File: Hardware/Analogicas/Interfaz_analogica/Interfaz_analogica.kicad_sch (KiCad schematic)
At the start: 1 part, among them U1 LM741

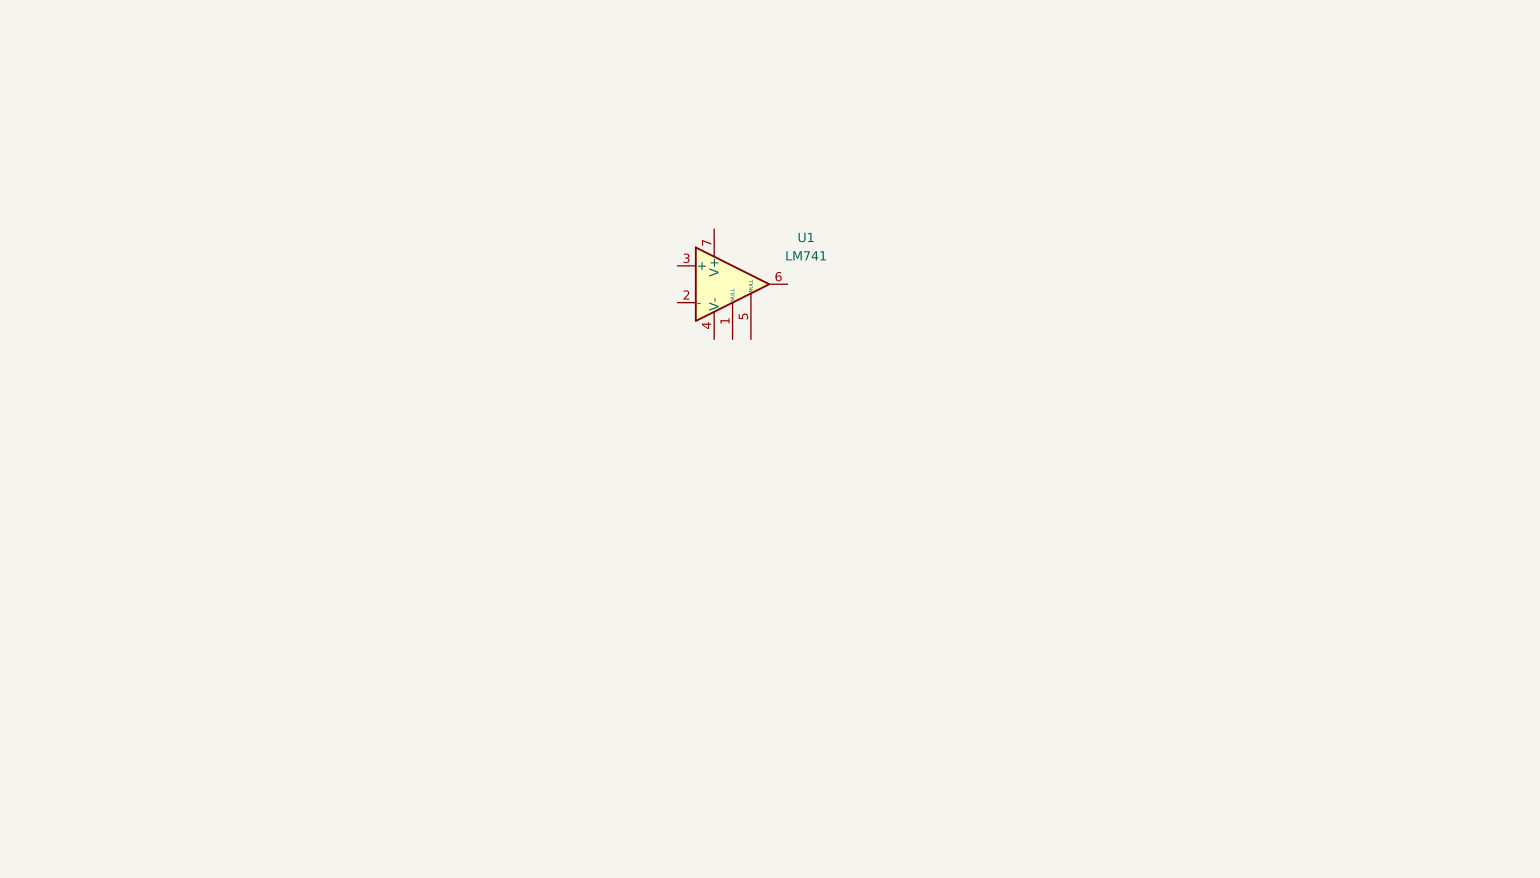
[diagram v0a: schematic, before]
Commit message: Interfaz analógica
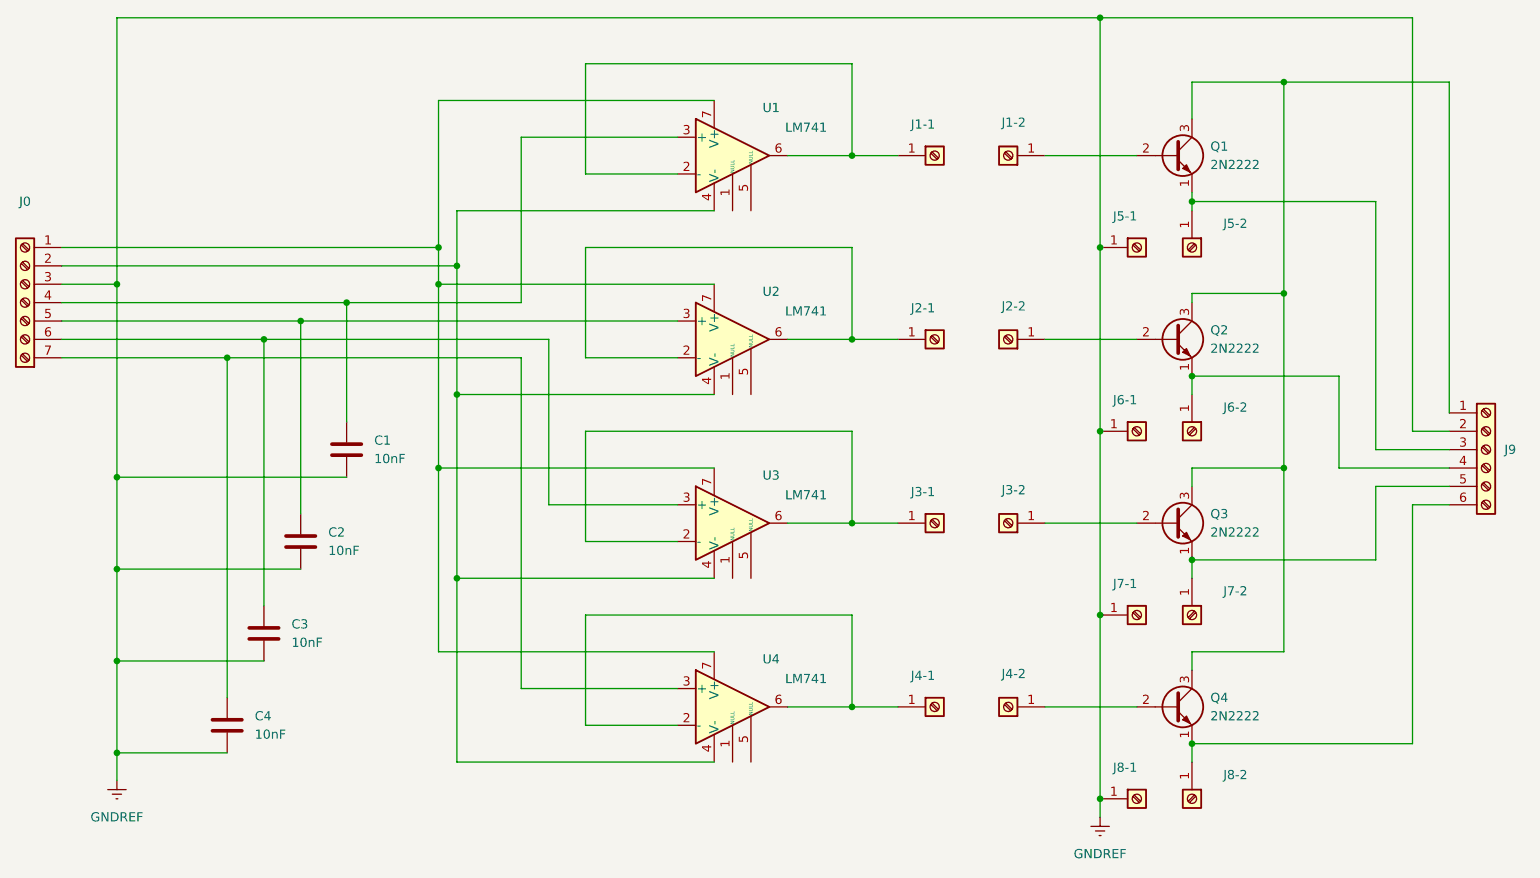
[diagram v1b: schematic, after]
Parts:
- added C1, C2, C3, C4: 10nF, symbol Device:C
- added J0: Screw_Terminal_01x07, symbol Connector:Screw_Terminal_01x07
- added J1-1, J1-2, J2-1, J2-2, J3-1, J3-2, J4-1, J4-2, J5-1, J5-2, J6-1, J6-2, J7-1, J7-2, J8-1, J8-2: Screw_Terminal_01x01, symbol Connector:Screw_Terminal_01x01
- added J9: Screw_Terminal_01x06, symbol Connector:Screw_Terminal_01x06
- added Q1, Q2, Q3, Q4: 2N2222, Package_TO_SOT_THT:TO-39-3, symbol Transistor_BJT:2N2219
- added U2, U3, U4: LM741, symbol Amplifier_Operational:LM741
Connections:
- net at U1.2 (-): now also U1.6, J1-1.1 (Pin_1)
- net at U1.3 (+): now also C1.1, J0.4 (Pin_4)
- net at U1.4 (V-): now also J0.2 (Pin_2), U2.4 (V-), U3.4 (V-), U4.4 (V-)
- net at U1.7 (V+): now also J0.1 (Pin_1), U2.7 (V+), U3.7 (V+), U4.7 (V+)
- new net: J6-2.1 (Pin_1), J9.4 (Pin_4), Q2.1 (E)
- new net: J7-2.1 (Pin_1), J9.5 (Pin_5), Q3.1 (E)
- new net: C3.1, J0.6 (Pin_6), U3.3 (+)
- new net: J3-1.1 (Pin_1), U3.2 (-), U3.6
- new net: J4-1.1 (Pin_1), U4.2 (-), U4.6
- new net: C4.1, J0.7 (Pin_7), U4.3 (+)
- new net: J2-1.1 (Pin_1), U2.2 (-), U2.6
- new net: C2.1, J0.5 (Pin_5), U2.3 (+)
- new net: J2-2.1 (Pin_1), Q2.2 (B)
- new net: J9.1 (Pin_1), Q1.3 (C), Q2.3 (C), Q3.3 (C), Q4.3 (C)
- new net: J5-2.1 (Pin_1), J9.3 (Pin_3), Q1.1 (E)
- new net: J8-2.1 (Pin_1), J9.6 (Pin_6), Q4.1 (E)
- new net: J4-2.1 (Pin_1), Q4.2 (B)
- new net: J3-2.1 (Pin_1), Q3.2 (B)
- new net: J1-2.1 (Pin_1), Q1.2 (B)
- new net GNDREF: C1.2, C2.2, C3.2, C4.2, J0.3 (Pin_3), J5-1.1 (Pin_1), J6-1.1 (Pin_1), J7-1.1 (Pin_1), J8-1.1 (Pin_1), J9.2 (Pin_2)
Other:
- moved on the sheet: U1
